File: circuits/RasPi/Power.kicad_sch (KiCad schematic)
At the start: 71 parts, among them IC1 DCDC_MPM3620A, J6 USB_C_Receptacle_USB2.0, Q10 BSS138, Q11 SSM3J332R, Q12 SSM6J808R, Q13 BSS138, Q14 SSM6J808R, Q15 S8550, Q16 SSM3J332R, Q17 S8550, Q6 SSM3J332R, Q7 S8550, Q8 SSM3J332R, Q9 S8550, SW4 SW_SPDT_White

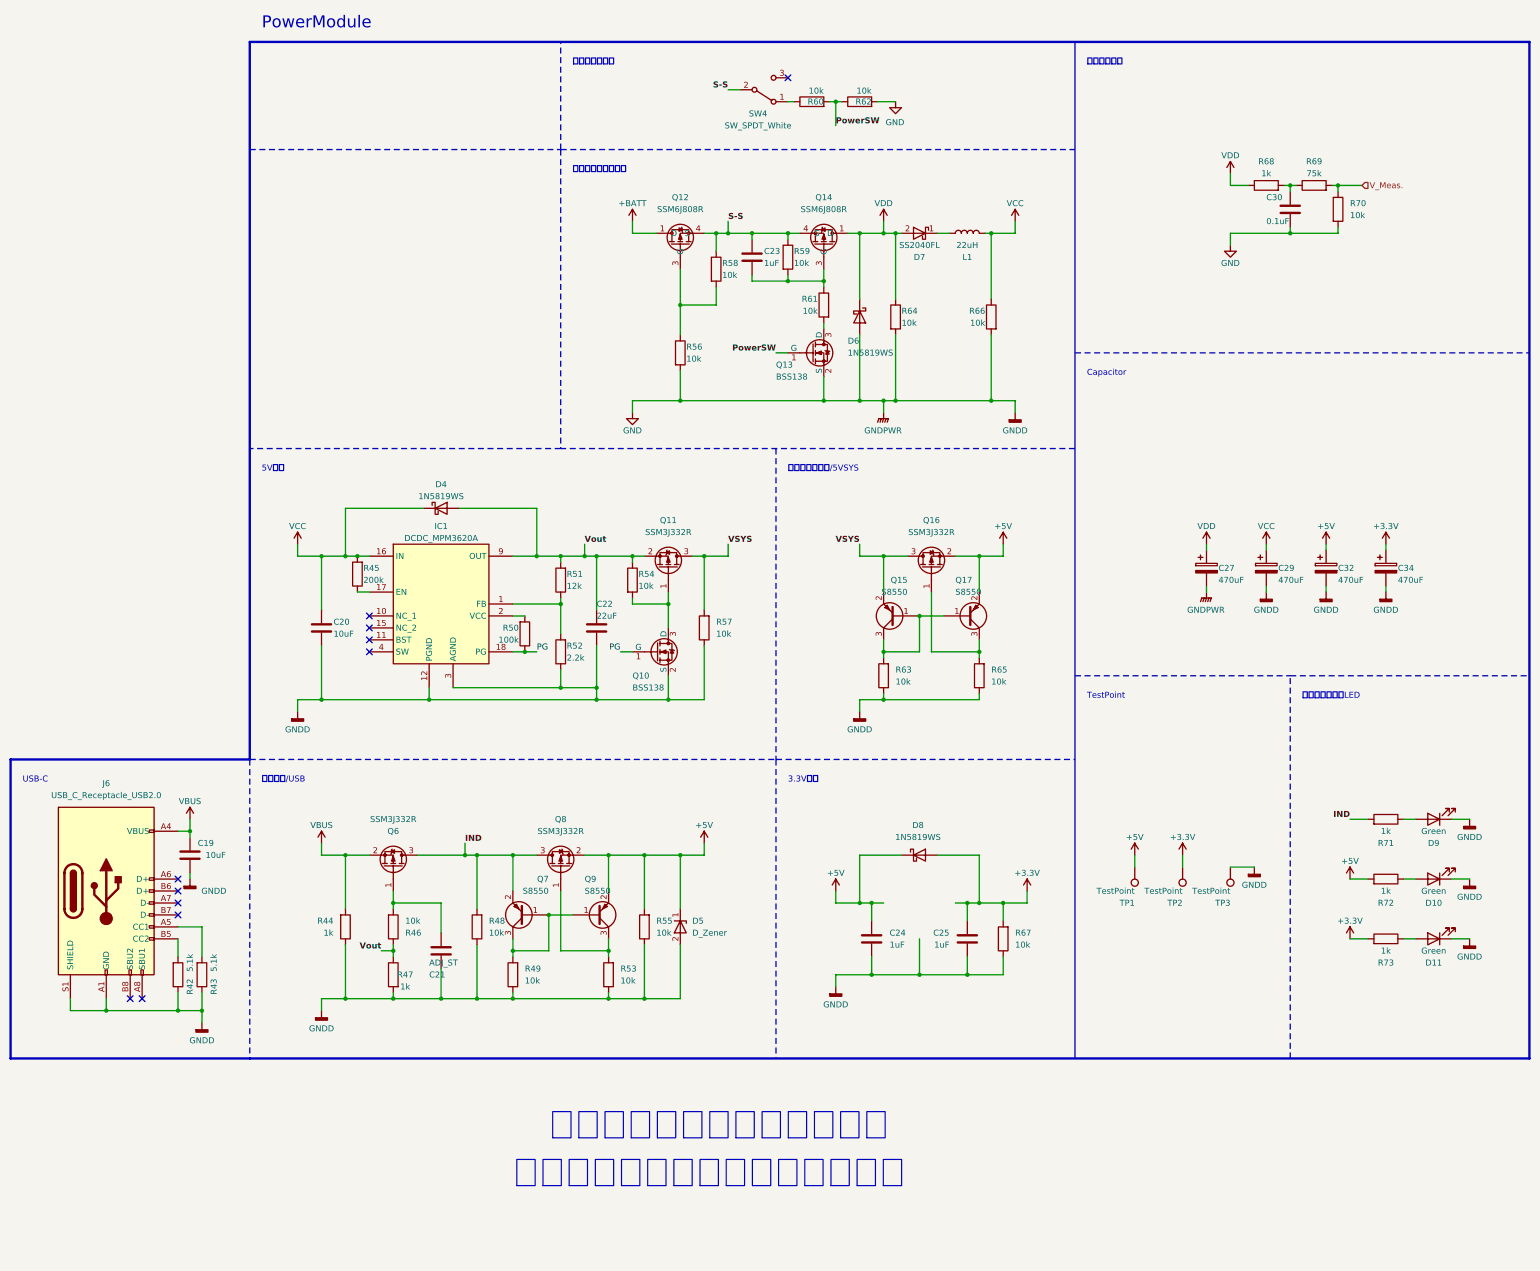
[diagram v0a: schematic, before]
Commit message: PDFプロット
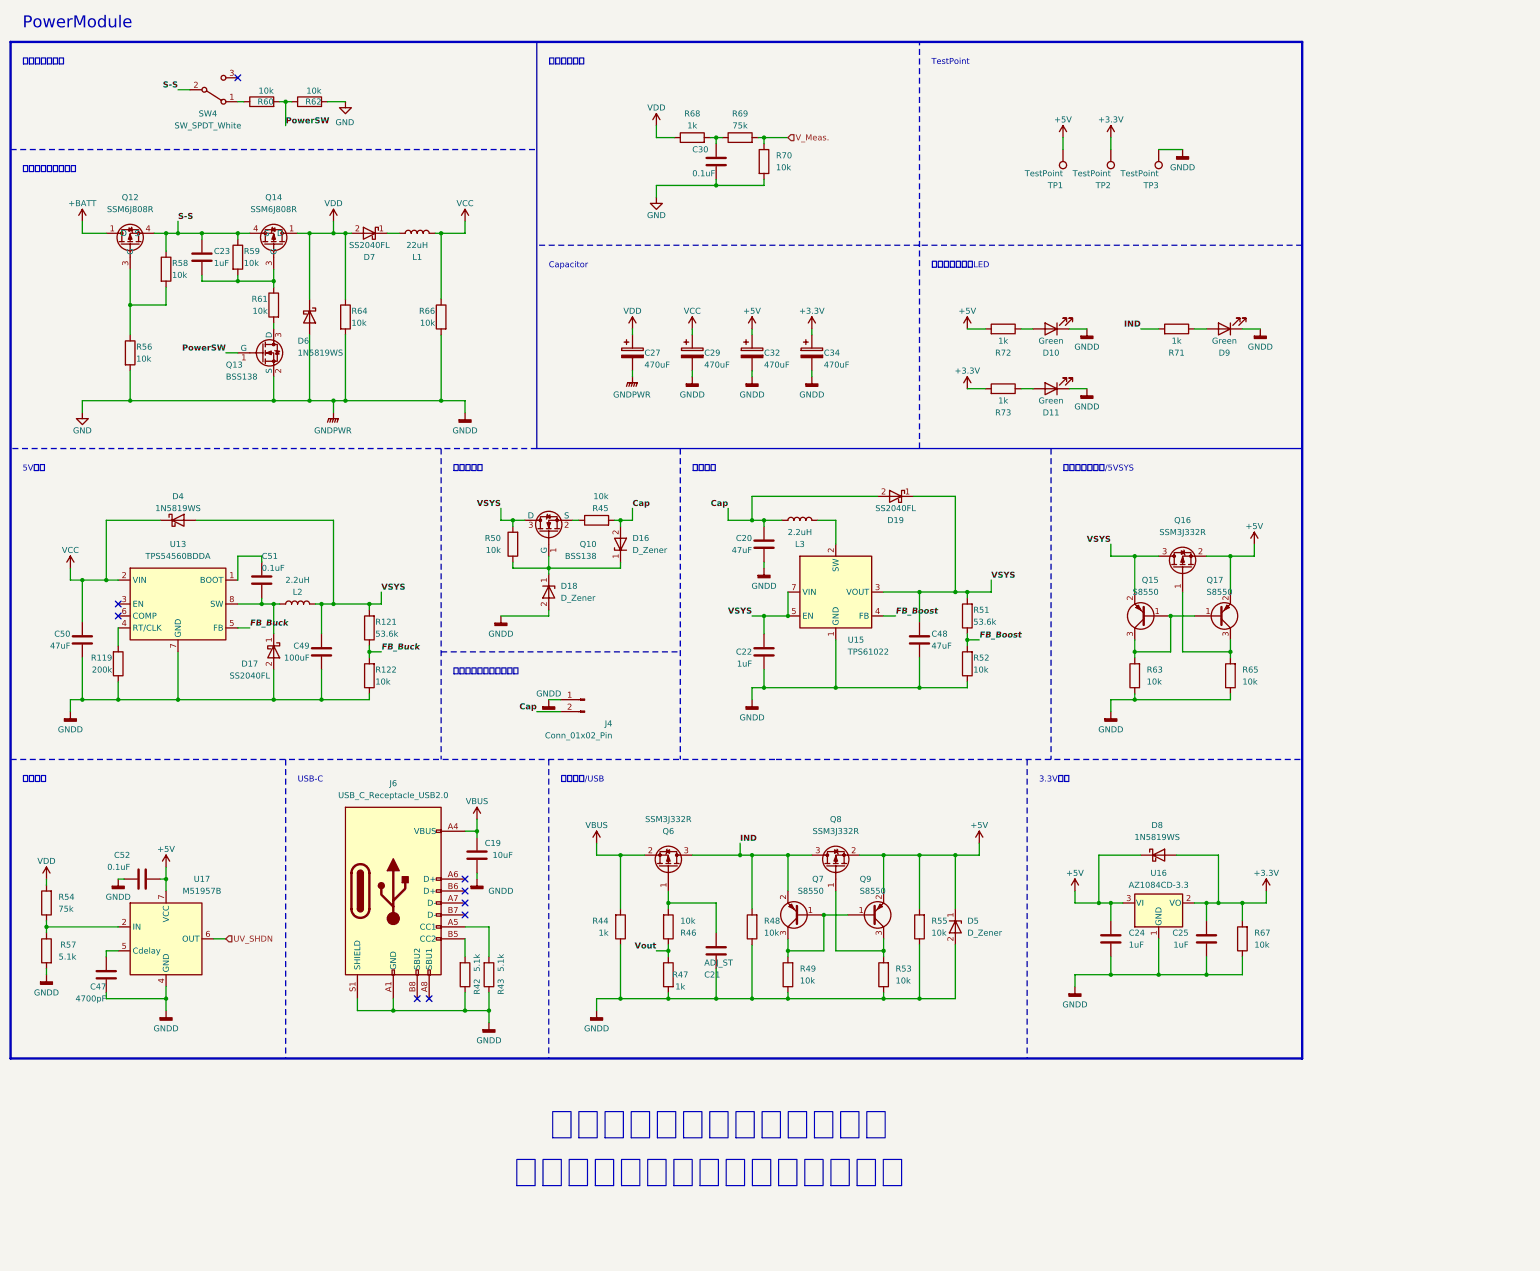
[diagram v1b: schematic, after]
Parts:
- removed IC1: DCDC_MPM3620A, MyLibrary:DCDC_MPM3620A, symbol MyLibrary:DCDC_MPM3620A
- removed Q11: SSM3J332R, Package_TO_SOT_SMD:SOT-23W, symbol Device:Q_PMOS_GSD
- added C47: 4700pF, Capacitor_SMD:C_0603_1608Metric, symbol Device:C
- added C48, C50: 47uF, Capacitor_SMD:C_0805_2012Metric, symbol Device:C
- added C49: 100uF, Capacitor_SMD:C_0805_2012Metric, symbol Device:C
- added C51: 0.1uF, Capacitor_SMD:C_0603_1608Metric, symbol Device:C
- added C52: 0.1uF, Capacitor_SMD:C_0402_1005Metric, symbol Device:C
- added D16, D18: D_Zener, Diode_SMD:D_SOD-323_HandSoldering, symbol Device:D_Zener
- added D17, D19: SS2040FL, Diode_SMD:D_SOD-123, symbol Device:D_Schottky
- added J4: Conn_01x02_Pin, symbol Connector:Conn_01x02_Pin
- added L2, L3: 2.2uH, MyLibrary:Inductor_CDPH4D19F, symbol Device:L
- added R119: 200k, Resistor_SMD:R_0402_1005Metric, symbol Device:R
- added R121: 53.6k, Resistor_SMD:R_0402_1005Metric, symbol Device:R
- added R122: 10k, Resistor_SMD:R_0402_1005Metric, symbol Device:R
- added U13: TPS54560BDDA, Package_SO:Texas_R-PDSO-G8_EP2.95x4.9mm_Mask2.4x3.1mm_ThermalVias, symbol Regulator_Switching:TPS54560BDDA
- added U15: TPS61022, Package_DFN_QFN:Texas_RWU0007A_VQFN-7_2x2mm_P0.5mm, symbol Converter_DCDC:TPS61022
- added U16: AZ1084CD-3.3, Package_TO_SOT_SMD:TO-252-2, symbol Regulator_Linear:AMS1117CD-3.3
- added U17: M51957B, Package_SO:SOP-8_3.9x4.9mm_P1.27mm, symbol Voltage_Supervisor:M51957B
- C20: value 10uF -> 47uF; footprint Capacitor_SMD:C_1206_3216Metric -> Capacitor_SMD:C_0805_2012Metric
- C22: value 22uF -> 1uF; footprint Capacitor_SMD:C_0805_2012Metric -> Capacitor_SMD:C_0603_1608Metric
- R45: value 200k -> 10k
- R50: value 100k -> 10k
- R51: value 12k -> 53.6k
- R52: value 2.2k -> 10k
- R54: value 10k -> 75k; footprint Resistor_SMD:R_0402_1005Metric -> Resistor_SMD:R_0603_1608Metric
- R57: value 10k -> 5.1k; footprint Resistor_SMD:R_0402_1005Metric -> Resistor_SMD:R_0603_1608Metric
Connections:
- net +3.3V: now also U16.2 (VO)
- net +5V: now also C52.2, U16.3 (VI), U17.7 (VCC)
- net GND: now also R57.2, C47.1, C48.2, C49.2, C50.2, C52.1, D17.2 (A), D18.2 (A), J4.1 (Pin_1), R119.1, R122.1, U13.7 (GND), U13.9 (GND), U15.1 (GND), U16.1 (GND), U17.4 (GND); no longer Q10.2 (S), R57.1
- net VCC: now also C50.1, U13.2 (VIN); no longer C20.1, R45.2
- net VDD: now also R54.2
- net VSYS: now also C22.1, D4.2 (A), Q10.3 (D), R50.2, R51.2, C48.1, C49.1, D19.1 (K), L2.2, R121.2, U15.3 (VOUT), U15.5 (EN), U15.7 (VIN); no longer R57.2
- net Vout: no longer C22.1, D4.2 (A), R51.2, R54.1
- net FB_Boost: now reaches R51.1, R52.2
- net FB_Boost: now also U15.4 (FB)
- net at R45.1: now also Q10.2 (S)
- net PG: no longer names the net of Q10.1 (G), R50.1
- net PG: now also D16.1 (K), D18.1 (K)
- new net: R54.1, R57.1, U17.2 (IN)
- new net: C47.2, U17.5 (Cdelay)
- new net: C51.2, D17.1 (K), L2.1, U13.8 (SW)
- new net: L3.1, U15.2 (SW)
- new net: C51.1, U13.1 (BOOT)
- new net: R119.2, U13.4 (RT/CLK)
- new net Cap: C20.1, D16.2 (A), D19.2 (A), J4.2 (Pin_2), L3.2, R45.2
- new net FB_Buck: R121.1, R122.2, U13.5 (FB)
- new net UV_SHDN: U17.6 (OUT)
- no-connect marks 11 -> 9
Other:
- note added: "定電流回路"
- note added: "昇圧回路"
- note added: "電圧監視"
- note added: "電気二重層キャパシタへ"
- moved on the sheet: C19, C21, C23, C24, C25, C27, C29, C30, C32, C34, D10, D11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

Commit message: panelフットプリント配置
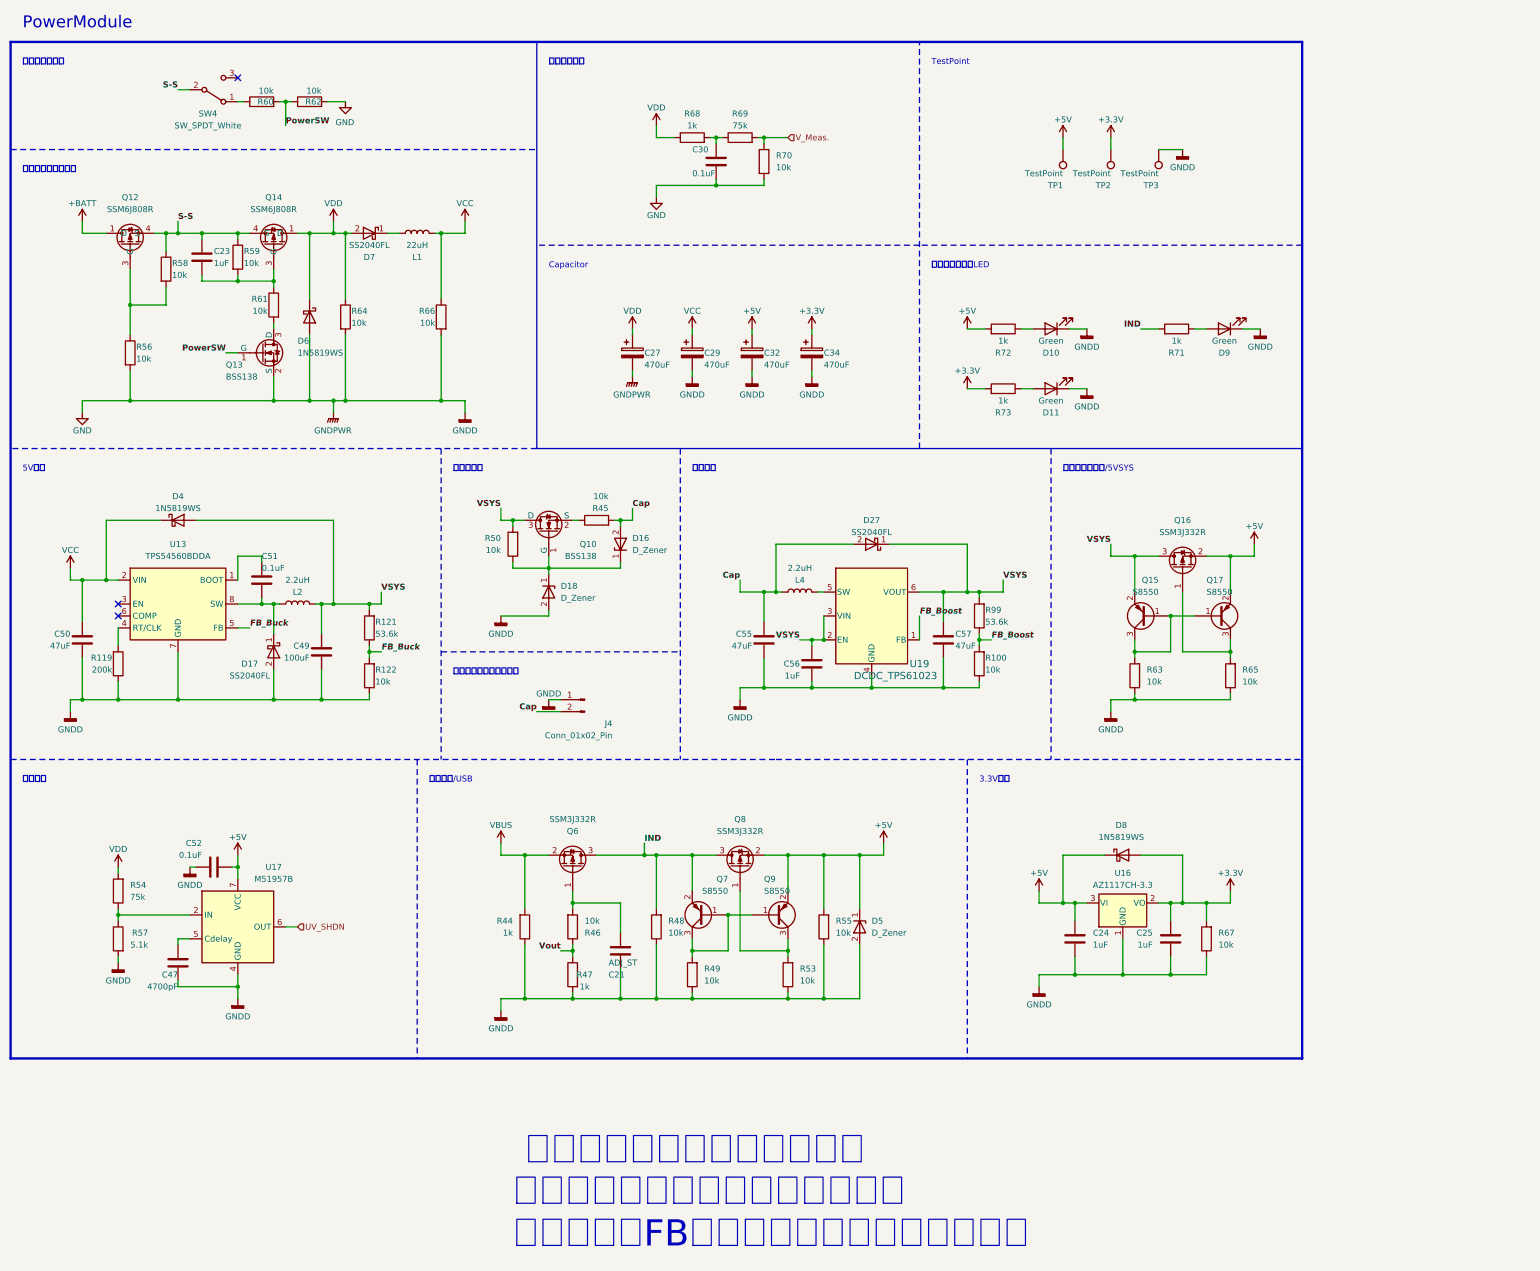
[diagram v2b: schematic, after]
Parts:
- removed C19: 10uF, Capacitor_SMD:C_0805_2012Metric, symbol Device:C
- removed C20, C48: 47uF, Capacitor_SMD:C_0805_2012Metric, symbol Device:C
- removed C22: 1uF, Capacitor_SMD:C_0603_1608Metric, symbol Device:C
- removed D19: SS2040FL, Diode_SMD:D_SOD-123, symbol Device:D_Schottky
- removed J6: USB_C_Receptacle_USB2.0, Connector_USB:USB_C_Receptacle_G-Switch_GT-USB-7010ASV, symbol Connector:USB_C_Receptacle_USB2.0
- removed L3: 2.2uH, MyLibrary:Inductor_CDPH4D19F, symbol Device:L
- removed R42, R43: 5.1k, Resistor_SMD:R_0402_1005Metric, symbol Device:R
- removed R51: 53.6k, Resistor_SMD:R_0402_1005Metric, symbol Device:R
- removed R52: 10k, Resistor_SMD:R_0402_1005Metric, symbol Device:R
- removed U15: TPS61022, Package_DFN_QFN:Texas_RWU0007A_VQFN-7_2x2mm_P0.5mm, symbol Converter_DCDC:TPS61022
- added C55, C57: 47uF, Capacitor_SMD:C_0805_2012Metric, symbol Device:C
- added C56: 1uF, Capacitor_SMD:C_0603_1608Metric, symbol Device:C
- added D27: SS2040FL, Diode_SMD:D_SOD-123, symbol Device:D_Schottky
- added L4: 2.2uH, MyLibrary:Inductor_CDPH4D19F, symbol Device:L
- added R100: 10k, Resistor_SMD:R_0402_1005Metric, symbol Device:R
- added R99: 53.6k, Resistor_SMD:R_0402_1005Metric, symbol Device:R
- added U19: DCDC_TPS61023, MyLibrary:DCDC_TPS61023, symbol MyLibrary:DCDC_TPS61023
- U16: value AZ1084CD-3.3 -> AZ1117CH-3.3; footprint Package_TO_SOT_SMD:TO-252-2 -> Package_TO_SOT_SMD:SOT-223-3_TabPin2
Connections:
- net Cap: now also C55.1, D27.2 (A), L4.2
- net FB_Boost: now also R100.2, R99.1, U19.1 (FB)
- net GND: now also C55.2, C56.2, C57.2, R100.1, U19.4 (GND)
- net VSYS: now also C56.1, C57.1, D27.1 (K), R99.2, U19.2 (EN), U19.3 (VIN), U19.6 (VOUT)
- new net: L4.1, U19.5 (SW)
- no-connect marks 9 -> 3
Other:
- note added: "三端子を新しく選定したのにする 昇圧回路のFB電圧をちょっと低く設定する"
- note removed: "USB-C"
- note removed: "三端子を新しく選定したのにする"
- moved on the sheet: C21, C24, C25, C47, C52, D5, D8, Q6, Q7, Q8, Q9, R44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
